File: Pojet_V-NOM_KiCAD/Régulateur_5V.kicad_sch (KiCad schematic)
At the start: 15 parts, among them IC1 MP1475SGJ-P

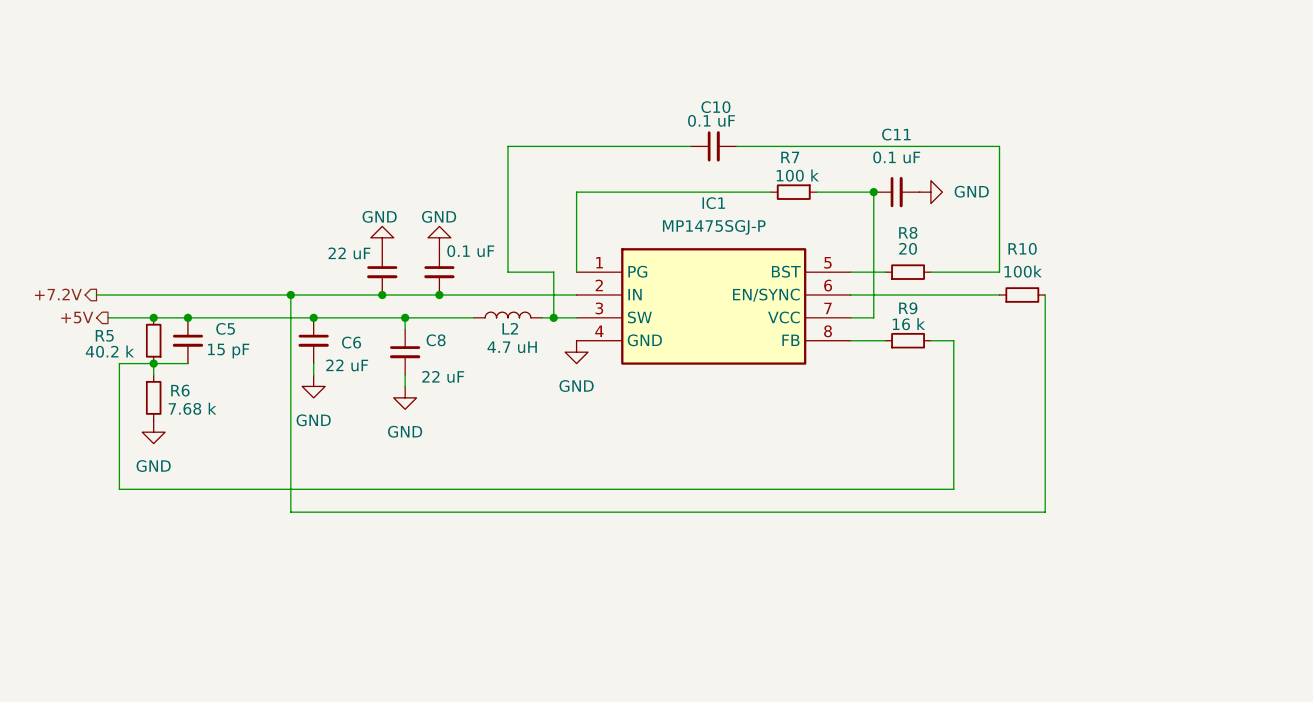
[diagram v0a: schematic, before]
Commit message: Maj
Maj lidar et regualteur
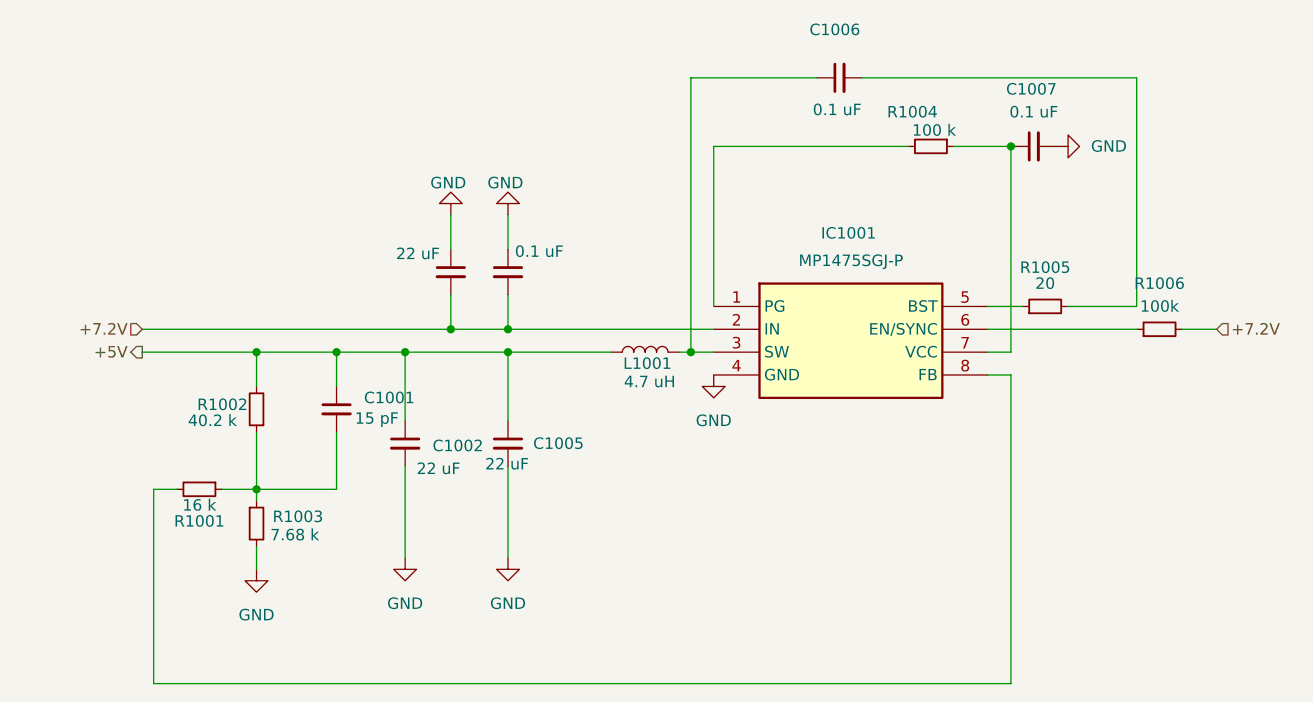
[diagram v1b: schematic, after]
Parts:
- removed C10, C11, C9: 0.1 uF, symbol Device:C_Small
- removed C5: 15 pF, symbol Device:C_Small
- removed C6, C7, C8: 22 uF, symbol Device:C_Small
- removed IC1: MP1475SGJ-P, SOT65P280X100-8N, symbol MP1475SGJ-P:MP1475SGJ-P
- removed L2: 4.7 uH, symbol Device:L
- removed R10: 100k, symbol Device:R_Small
- removed R5: 40.2 k, symbol Device:R_Small
- removed R6: 7.68 k, symbol Device:R_Small
- removed R7: 100 k, symbol Device:R_Small
- removed R8: 20, symbol Device:R_Small
- removed R9: 16 k, symbol Device:R_Small
- added C1001: 15 pF, symbol Device:C_Small
- added C1002, C1003, C1005: 22 uF, symbol Device:C_Small
- added C1004, C1006, C1007: 0.1 uF, symbol Device:C_Small
- added IC1001: MP1475SGJ-P, SOT65P280X100-8N, symbol MP1475SGJ-P:MP1475SGJ-P
- added L1001: 4.7 uH, symbol Device:L
- added R1001: 16 k, symbol Device:R_Small
- added R1002: 40.2 k, symbol Device:R_Small
- added R1003: 7.68 k, symbol Device:R_Small
- added R1004: 100 k, symbol Device:R_Small
- added R1005: 20, symbol Device:R_Small
- added R1006: 100k, symbol Device:R_Small
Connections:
- net +5V: now also C1001.1, C1002.1, C1005.1, L1001.1, R1002.2
- net +7.2V: now also C1003.2, C1004.2, IC1001.2 (IN), R1006.2
- net GND: now also C1002.2, C1003.1, C1004.1, C1005.2, C1007.2, IC1001.4 (GND), R1003.2
- new net: C1001.2, R1001.1, R1002.1, R1003.1
- new net: IC1001.8 (FB), R1001.2
- new net: C1006.1, IC1001.3 (SW), L1001.2
- new net: C1006.2, R1005.2
- new net: IC1001.5 (BST), R1005.1
- new net: IC1001.1 (PG), R1004.2
- new net: IC1001.6 (EN/SYNC), R1006.1
- new net: C1007.1, IC1001.7 (VCC), R1004.1
